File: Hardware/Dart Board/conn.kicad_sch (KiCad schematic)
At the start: 2 parts, among them J1 Conn_01x20_Socket, J2 Conn_01x20_Socket

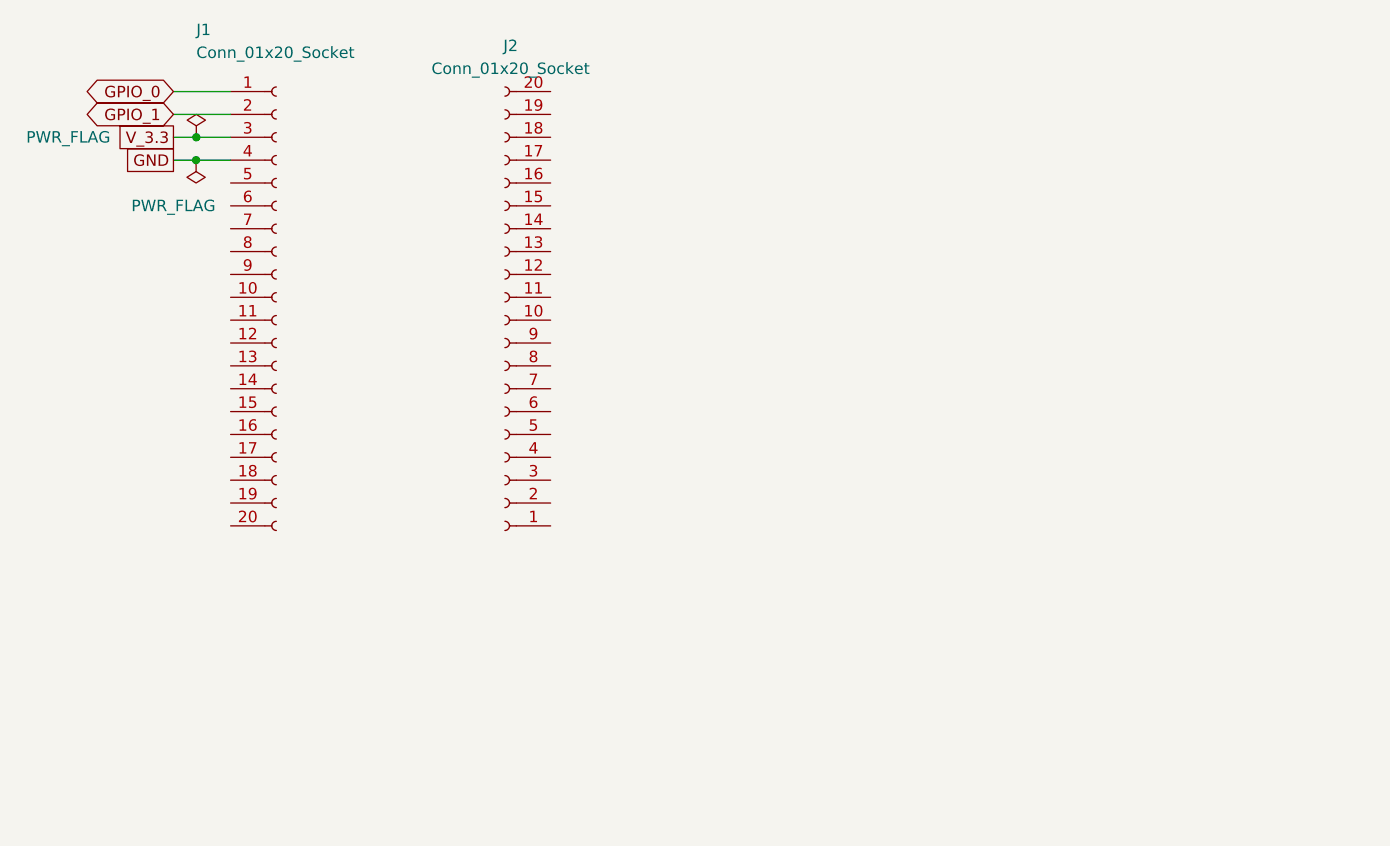
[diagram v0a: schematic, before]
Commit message: Piezo circuit
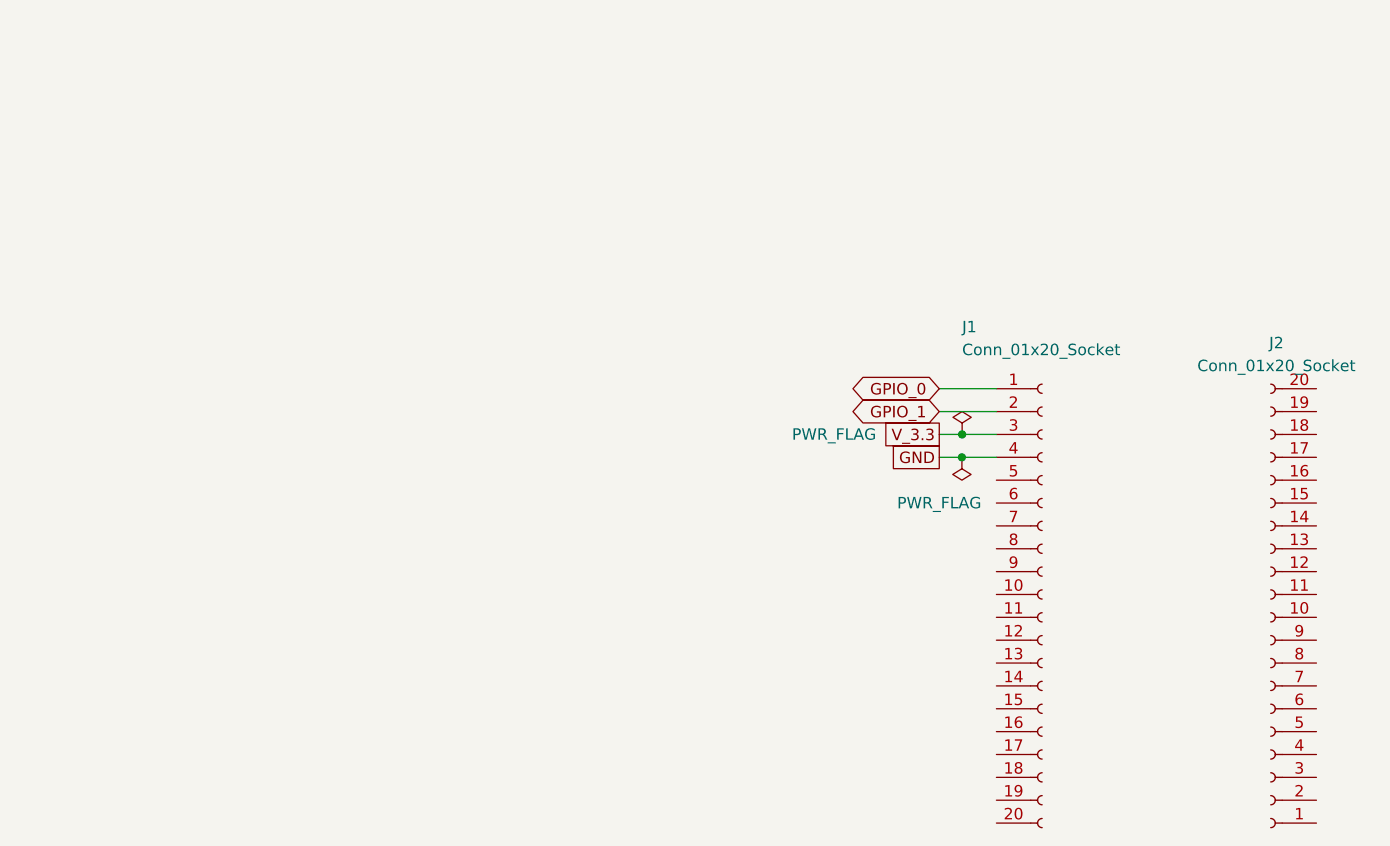
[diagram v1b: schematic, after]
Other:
- moved on the sheet: J1, J2
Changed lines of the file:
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@@
 	)
 	(junction
-		(at 33.02 40.64)
+		(at 118.11 73.66)
 		(diameter 0)
 		(color 0 0 0 0)
 	)
 	(junction
-		(at 32.9955 43.18)
+		(at 118.0855 76.2)
 		(diameter 0)
 		(color 0 0 0 0)
@@
 	(wire
 		(pts
-			(xy 30.48 35.56) (xy 36.83 35.56)
-		)
-		(stroke
-			(width 0)
-			(type default)
-		)
-	)
-	(wire
-		(pts
-			(xy 33.02 40.64) (xy 36.83 40.64)
-		)
-		(stroke
-			(width 0)
-			(type default)
-		)
-	)
-	(wire
-		(pts
-			(xy 30.48 40.64) (xy 33.02 40.64)
-		)
-		(stroke
-			(width 0)
-			(type default)
-		)
-	)
-	(wire
-		(pts
-			(xy 32.9955 43.18) (xy 36.83 43.18)
-		)
-		(stroke
-			(width 0)
-			(type default)
-		)
-	)
-	(wire
-		(pts
-			(xy 30.48 43.18) (xy 32.9955 43.18)
-		)
-		(stroke
-			(width 0)
-			(type default)
-		)
-	)
-	(wire
-		(pts
-			(xy 30.48 38.1) (xy 36.83 38.1)
+			(xy 115.57 68.58) (xy 121.92 68.58)
+		)
+		(stroke
+			(width 0)
+			(type default)
+		)
+	)
+	(wire
+		(pts
+			(xy 118.11 73.66) (xy 121.92 73.66)
+		)
+		(stroke
+			(width 0)
+			(type default)
+		)
+	)
+	(wire
+		(pts
+			(xy 115.57 73.66) (xy 118.11 73.66)
+		)
+		(stroke
+			(width 0)
+			(type default)
+		)
+	)
+	(wire
+		(pts
+			(xy 118.0855 76.2) (xy 121.92 76.2)
+		)
+		(stroke
+			(width 0)
+			(type default)
+		)
+	)
+	(wire
+		(pts
+			(xy 115.57 76.2) (xy 118.0855 76.2)
+		)
+		(stroke
+			(width 0)
+			(type default)
+		)
+	)
+	(wire
+		(pts
+			(xy 115.57 71.12) (xy 121.92 71.12)
 		)
 		(stroke
@@
 	(global_label "GPIO_0"
 		(shape bidirectional)
-		(at 30.48 35.56 180)
+		(at 115.57 68.58 180)
 		(fields_autoplaced yes)
 		(effects
@@
 		)
 		(property "Intersheetrefs" "${INTERSHEET_REFS}"
-			(at 19.7311 35.56 0)
+			(at 104.8211 68.58 0)
 			(effects
 				(font
@@
 	(global_label "GND"
 		(shape passive)
-		(at 30.48 43.18 180)
+		(at 115.57 76.2 180)
 		(fields_autoplaced yes)
 		(effects
@@
 		)
 		(property "Intersheetrefs" "${INTERSHEET_REFS}"
-			(at 24.7356 43.18 0)
+			(at 109.8256 76.2 0)
 			(effects
 				(font
@@
 	(global_label "V_3.3"
 		(shape passive)
-		(at 30.48 40.64 180)
+		(at 115.57 73.66 180)
 		(fields_autoplaced yes)
 		(effects
@@
 		)
 		(property "Intersheetrefs" "${INTERSHEET_REFS}"
-			(at 23.5261 40.64 0)
+			(at 108.6161 73.66 0)
 			(effects
 				(font
@@
 	(global_label "GPIO_1"
 		(shape bidirectional)
-		(at 30.48 38.1 180)
+		(at 115.57 71.12 180)
 		(fields_autoplaced yes)
 		(effects
@@
 		)
 		(property "Intersheetrefs" "${INTERSHEET_REFS}"
-			(at 19.7311 38.1 0)
+			(at 104.8211 71.12 0)
 			(effects
 				(font
@@
 	(symbol
 		(lib_id "Connector:Conn_01x20_Socket")
-		(at 67.31 60.96 180)
+		(at 152.4 93.98 180)
 		(unit 1)
 		(exclude_from_sim no)
@@
 		(fields_autoplaced yes)
 		(property "Reference" "J2"
-			(at 67.945 30.48 0)
+			(at 153.035 63.5 0)
 			(effects
 				(font
@@
 		)
 		(property "Value" "Conn_01x20_Socket"
-			(at 67.945 33.02 0)
+			(at 153.035 66.04 0)
 			(effects
 				(font
@@
 		)
 		(property "Footprint" ""
-			(at 67.31 60.96 0)
+			(at 152.4 93.98 0)
 			(effects
 				(font
@@
 		)
 		(property "Datasheet" "~"
-			(at 67.31 60.96 0)
+			(at 152.4 93.98 0)
 			(effects
 				(font
@@
 		)
 		(property "Description" "Generic connector, single row, 01x20, script generated"
-			(at 67.31 60.96 0)
+			(at 152.4 93.98 0)
 			(effects
 				(font
@@
 	(symbol
 		(lib_id "power:PWR_FLAG")
-		(at 32.9955 43.18 180)
+		(at 118.0855 76.2 180)
 		(unit 1)
 		(exclude_from_sim no)
@@
 		(dnp no)
 		(property "Reference" "#FLG02"
-			(at 32.9955 45.085 0)
+			(at 118.0855 78.105 0)
 			(effects
 				(font
@@
 		)
 		(property "Value" "PWR_FLAG"
-			(at 30.48 48.26 0)
+			(at 115.57 81.28 0)
 			(effects
 				(font
@@
 		)
 		(property "Footprint" ""
-			(at 32.9955 43.18 0)
+			(at 118.0855 76.2 0)
 			(effects
 				(font
@@
 		)
 		(property "Datasheet" "~"
-			(at 32.9955 43.18 0)
+			(at 118.0855 76.2 0)
 			(effects
 				(font
@@
 		)
 		(property "Description" "Special symbol for telling ERC where power comes from"
-			(at 32.9955 43.18 0)
+			(at 118.0855 76.2 0)
 			(effects
 				(font
@@
 	(symbol
 		(lib_id "power:PWR_FLAG")
-		(at 33.02 40.64 0)
+		(at 118.11 73.66 0)
 		(unit 1)
 		(exclude_from_sim no)
@@
 		(dnp no)
 		(property "Reference" "#FLG01"
-			(at 33.02 38.735 0)
+			(at 118.11 71.755 0)
 			(effects
 				(font
@@
 		)
 		(property "Value" "PWR_FLAG"
-			(at 18.796 40.64 0)
+			(at 103.886 73.66 0)
 			(effects
 				(font
@@
 		)
 		(property "Footprint" ""
-			(at 33.02 40.64 0)
+			(at 118.11 73.66 0)
 			(effects
 				(font
@@
 		)
 		(property "Datasheet" "~"
-			(at 33.02 40.64 0)
+			(at 118.11 73.66 0)
 			(effects
 				(font
@@
 		)
 		(property "Description" "Special symbol for telling ERC where power comes from"
-			(at 33.02 40.64 0)
+			(at 118.11 73.66 0)
 			(effects
 				(font
@@
 	(symbol
 		(lib_id "Connector:Conn_01x20_Socket")
-		(at 41.91 58.42 0)
+		(at 127 91.44 0)
 		(unit 1)
 		(exclude_from_sim no)
@@
 		(dnp no)
 		(property "Reference" "J1"
-			(at 33.02 28.702 0)
+			(at 118.11 61.722 0)
 			(effects
 				(font
@@
 		)
 		(property "Value" "Conn_01x20_Socket"
-			(at 33.02 31.242 0)
+			(at 118.11 64.262 0)
 			(effects
 				(font
@@
 		)
 		(property "Footprint" ""
-			(at 41.91 58.42 0)
+			(at 127 91.44 0)
 			(effects
 				(font
@@
 		)
 		(property "Datasheet" "~"
-			(at 41.91 58.42 0)
+			(at 127 91.44 0)
 			(effects
 				(font
@@
 		)
 		(property "Description" "Generic connector, single row, 01x20, script generated"
-			(at 41.91 58.42 0)
-			(effects
-				(font
+			(at 127 91.44 0)
+			(effects
+				(font
